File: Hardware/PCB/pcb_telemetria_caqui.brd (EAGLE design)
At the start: 105.2 x 104.1 mm, 34 parts

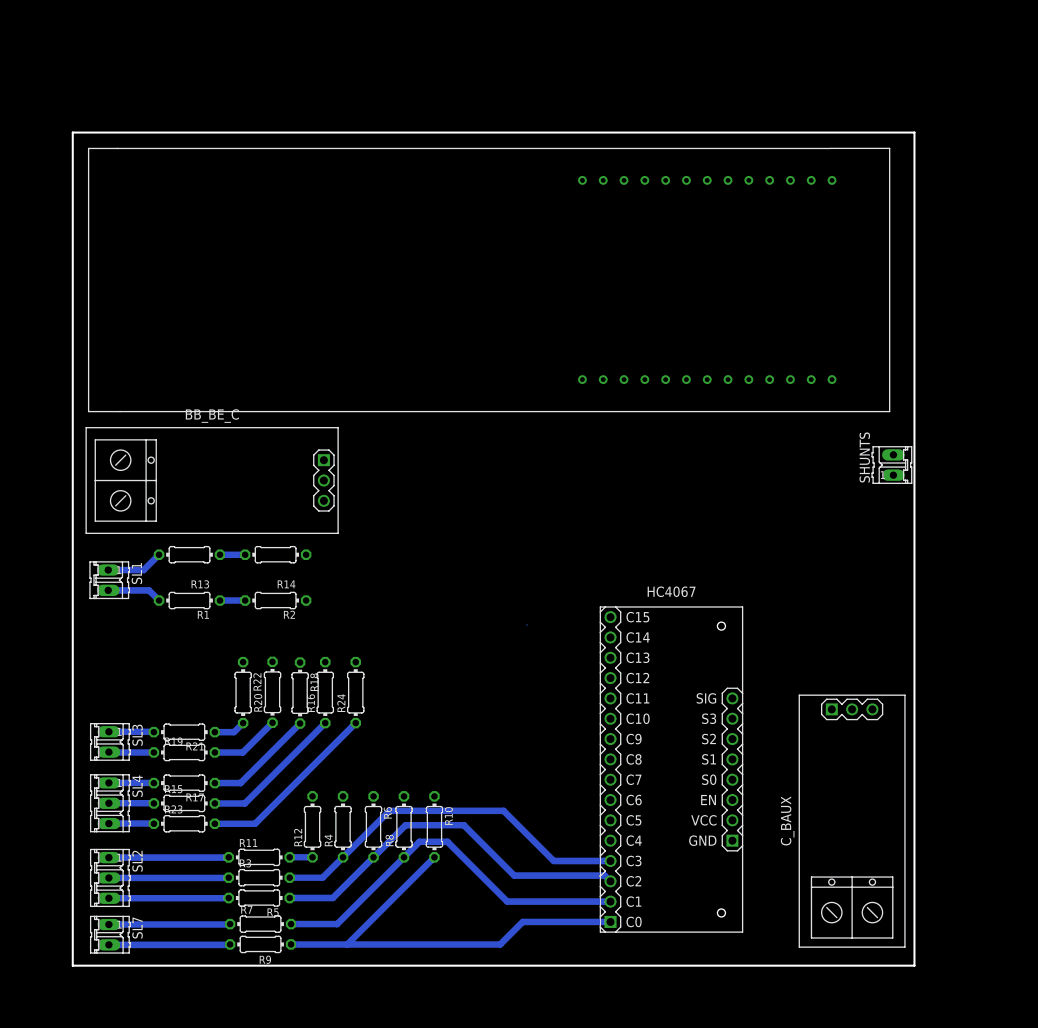
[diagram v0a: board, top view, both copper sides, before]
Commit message: uplix
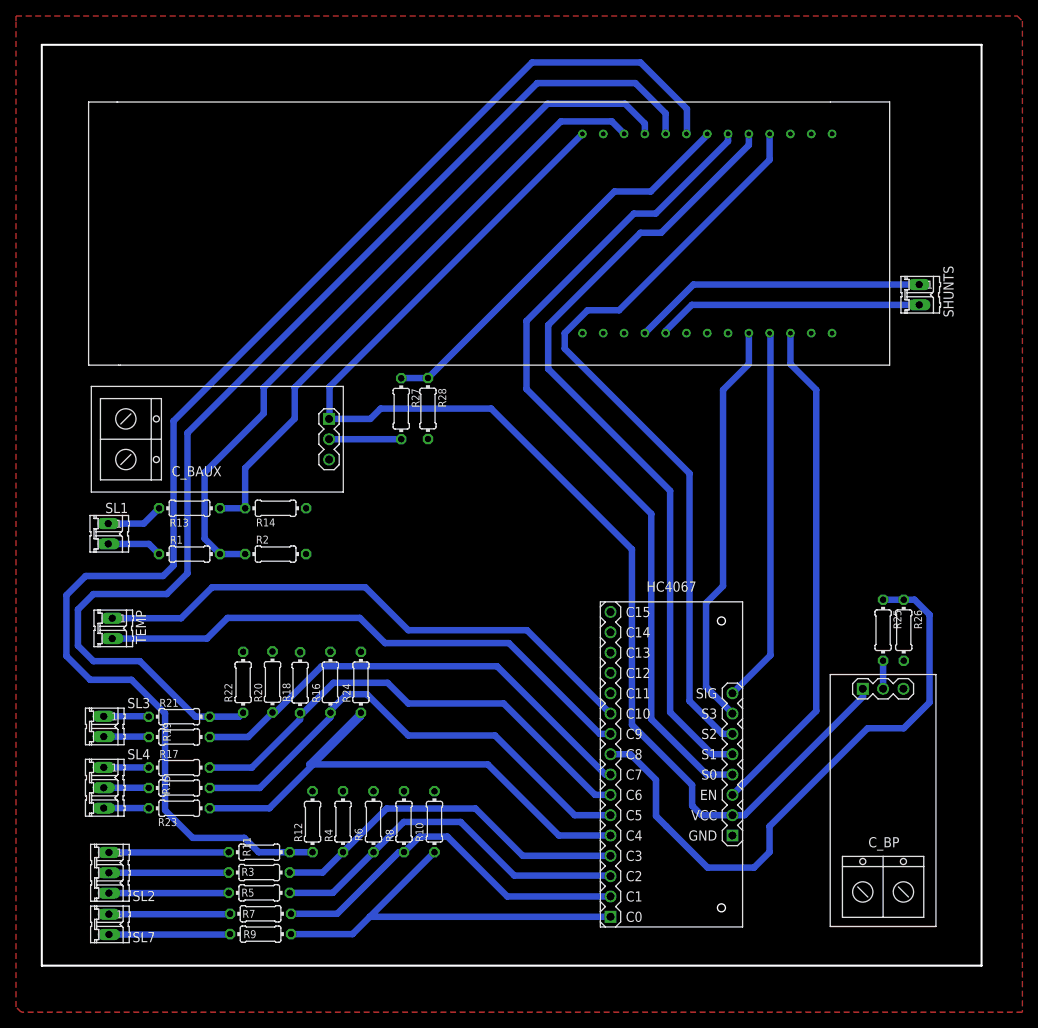
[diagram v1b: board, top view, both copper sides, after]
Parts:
- removed BB_BE_C: CURRENT-SENSOR-ACS712, diy-modules:CURRENT-SENSOR-ACS712
- added C_BP: CURRENT-SENSOR-ACS712, diy-modules:CURRENT-SENSOR-ACS712
- added R25, R27: 2.2k, rcl:0204/7
- added R26, R28: 3.9k, rcl:0204/7
- added TEMP: (no value), con-amp-quick:02P
- moved C_BAUX 92.6 mm to (18.1, 65.8), turned to 0 degrees
- moved SHUNTS 21.5 mm to (105.8, 83.9), turned to 270 degrees
- moved R1 5.81 mm to (14.6, 51.5)
- moved R13 5.81 mm to (14.6, 57.2)
- moved R14 5.81 mm to (25.4, 57.2)
- moved R2 5.81 mm to (25.4, 51.5)
- moved SL1 5.81 mm to (4.43, 54.0)
- moved U$1 5.81 mm to (78.7, 91.0)
- moved R15 2.04 mm to (13.3, 22.2)
- moved R17 2.04 mm to (13.3, 24.8)
- moved SL4 2.04 mm to (3.87, 22.2)
- moved SL3 2.04 mm to (3.87, 29.9)
- moved R19 2.04 mm to (13.3, 28.6)
- moved R21 2.04 mm to (13.3, 31.1)
- moved R23 2.04 mm to (13.3, 19.7)
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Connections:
- removed net EN: HC4067.J2.3
- removed net S0: HC4067.J2.4
- removed net S1: HC4067.J2.5
- removed net S2: HC4067.J2.6
- removed net S3: HC4067.J2.7
- removed net SIG: HC4067.J2.8
- removed net VCC: BB_BE_C.1, C_BAUX.1, HC4067.J2.2
- new net N$1: C_BP.2, R25.2
- new net N$2: C_BAUX.2, R27.2
- net 0: now also HC4067.J2.7
- net 13: now also R1.1, R2.2; no longer R23.2, R24.1
- net 14: now also R21.1, R22.2; no longer R13.1, R14.2
- net 2: now also R13.1, R14.2; no longer R11.2, R12.1
- net 21: now also SHUNTS.1; no longer SHUNTS.2
- net 22: now also SHUNTS.2; no longer SHUNTS.1
- net 23: now also HC4067.J2.3
- net 25: now also R11.2, R12.1; no longer R1.1, R2.2
- net 32: now also HC4067.J2.4
- net 33: now also R27.1, R28.1; no longer C_BAUX.2
- net 34: now also HC4067.J2.6
- net 35: now also HC4067.J2.5
- net 4: now also HC4067.J2.8
- net 5V: now also C_BAUX.1, C_BP.1, HC4067.J2.2
- net BAT_AUX: now also R21.2, SL3.1; no longer R23.1, SL4.3
- net C10: now also TEMP.1
- net C4: now also R23.2, R24.1; no longer R21.1, R22.2
- net C5: now also R15.2, R16.1; no longer R19.2, R20.1
- net C7: now also R19.2, R20.1; no longer R15.2, R16.1
- net C8: now also R25.1, R26.1
- net C9: now also TEMP.2
- net COOLER_E: now also R23.1, SL4.3; no longer R21.2, SL3.1
- net GND: now also C_BP.3, R26.2, R28.2; no longer BB_BE_C.3
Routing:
- net 25: track 3.14 -> 176.9 mm
- net 5V: track 0.00 -> 158.6 mm
- net 14: track 3.14 -> 144.2 mm
- net 32: track 0.00 -> 104.7 mm
- net 35: track 0.00 -> 100.5 mm
- net 34: track 0.00 -> 97.3 mm
- net C8: track 0.00 -> 76.4 mm
- net 2: track 2.85 -> 76.4 mm
- net C4: track 4.00 -> 74.6 mm
- net C10: track 0.00 -> 70.4 mm
- net 13: track 22.8 -> 92.5 mm
- net C9: track 0.00 -> 69.4 mm
- net 23: track 0.00 -> 63.4 mm
- net C5: track 8.75 -> 61.7 mm
- net 0: track 0.00 -> 51.1 mm
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- added copper zone on layer 1, net GND
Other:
- board size 105.2 x 104.1 mm -> 117.5 x 115.1 mm
